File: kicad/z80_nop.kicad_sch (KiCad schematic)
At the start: 36 parts, among them J1 USB_C_Receptacle_PowerOnly_6P, J2 USB_A, J5 Barrel_Jack, SW1 SW_Push, U1 LM555CN, U2 Z80

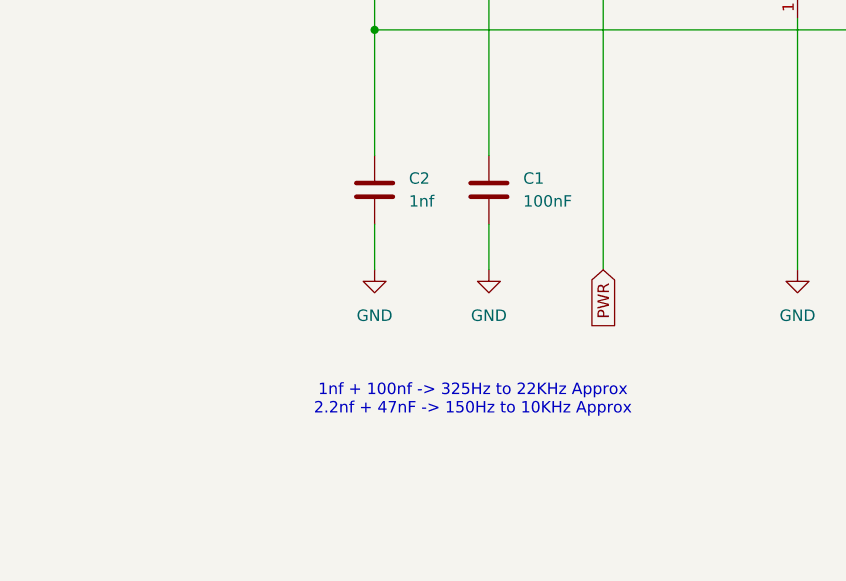
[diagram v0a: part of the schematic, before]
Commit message: Update docs
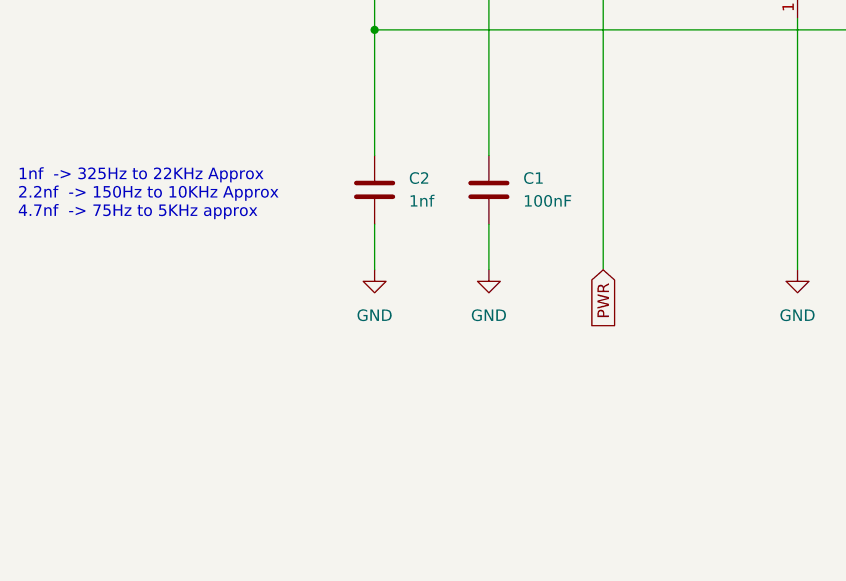
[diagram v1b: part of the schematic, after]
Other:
- note added: "1nf -> 325Hz to 22KHz Approx 2.2nf -> 150Hz to 10KHz Approx 4.7nf -> 75Hz to 5KHz approx"
- note removed: "1nf + 100nf -> 325Hz to 22KHz Approx 2.2nf + 47nF -> 150Hz to 10KHz Approx"
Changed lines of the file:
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@@
 		)
 	)
-	(text "1nf + 100nf -> 325Hz to 22KHz Approx\n2.2nf + 47nF -> 150Hz to 10KHz Approx"
+	(text "1nf  -> 325Hz to 22KHz Approx\n2.2nf  -> 150Hz to 10KHz Approx\n4.7nf  -> 75Hz to 5KHz approx\n"
 		(exclude_from_sim no)
-		(at 99.822 123.698 0)
+		(at 49.276 100.838 0)
 		(effects
 			(font
@@
 				(thickness 0.1588)
 			)
+			(justify left)
 		)
 	)
